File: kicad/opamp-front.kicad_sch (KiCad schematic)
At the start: 84 parts, among them J1 B+, J2 SPK, J3 INPUT, J4 GND, J5 B-, J6 GND, Q1 2N5551, Q10 2N2906, Q11 MJL3281C, Q12 2N2904, Q13 MJL1302C, Q2 BD139, Q3 BD140, Q4 BD139, Q5 BD139, Q6 2N5401, Q7 2N5551, Q8 2N5401, Q9 BD140, U1 LM4562

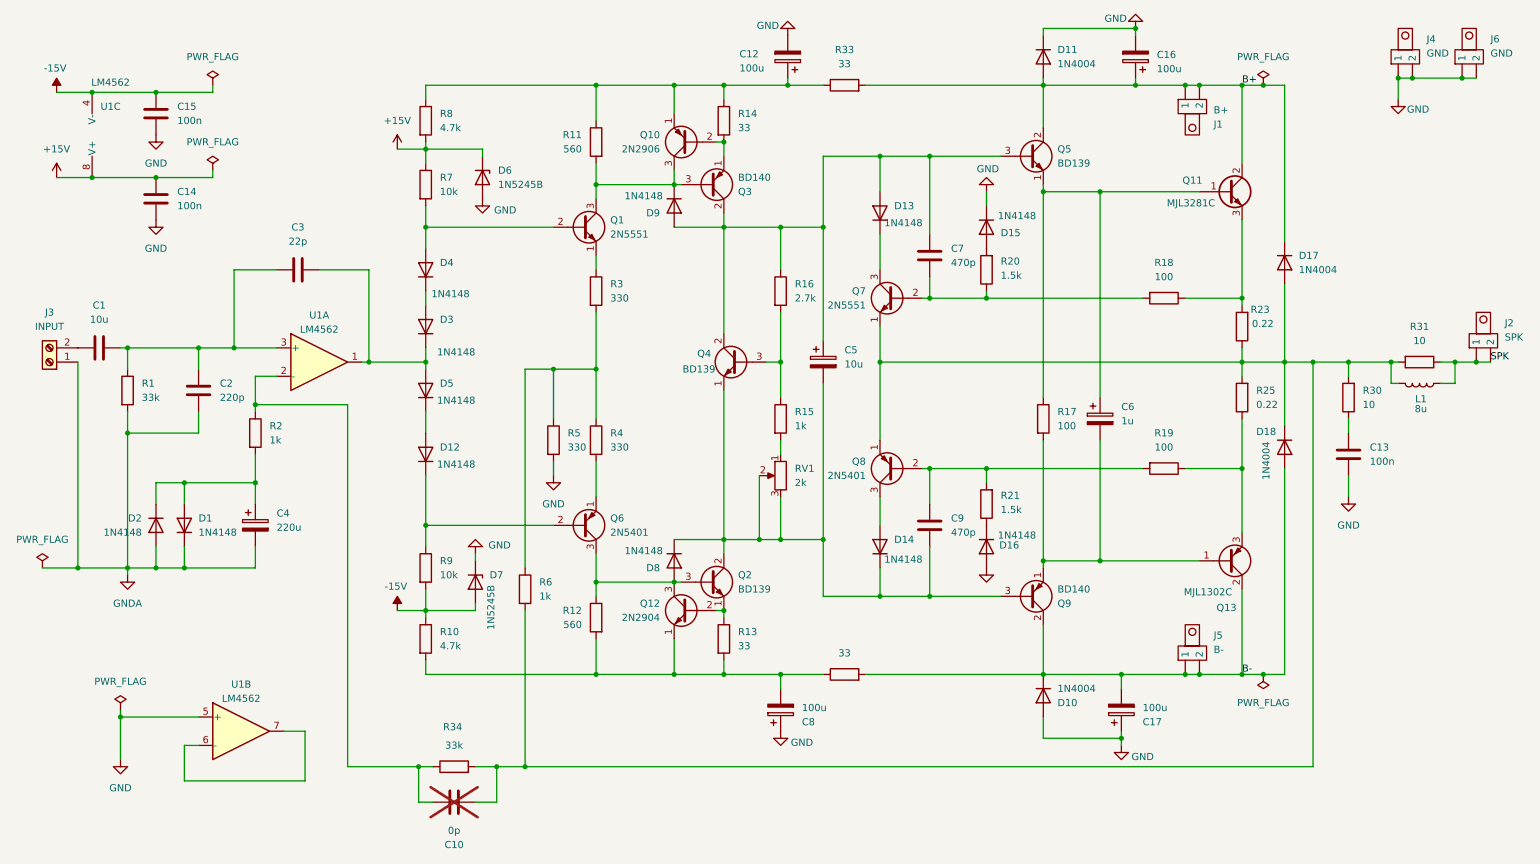
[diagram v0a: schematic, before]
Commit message: Restored after rebase mishap
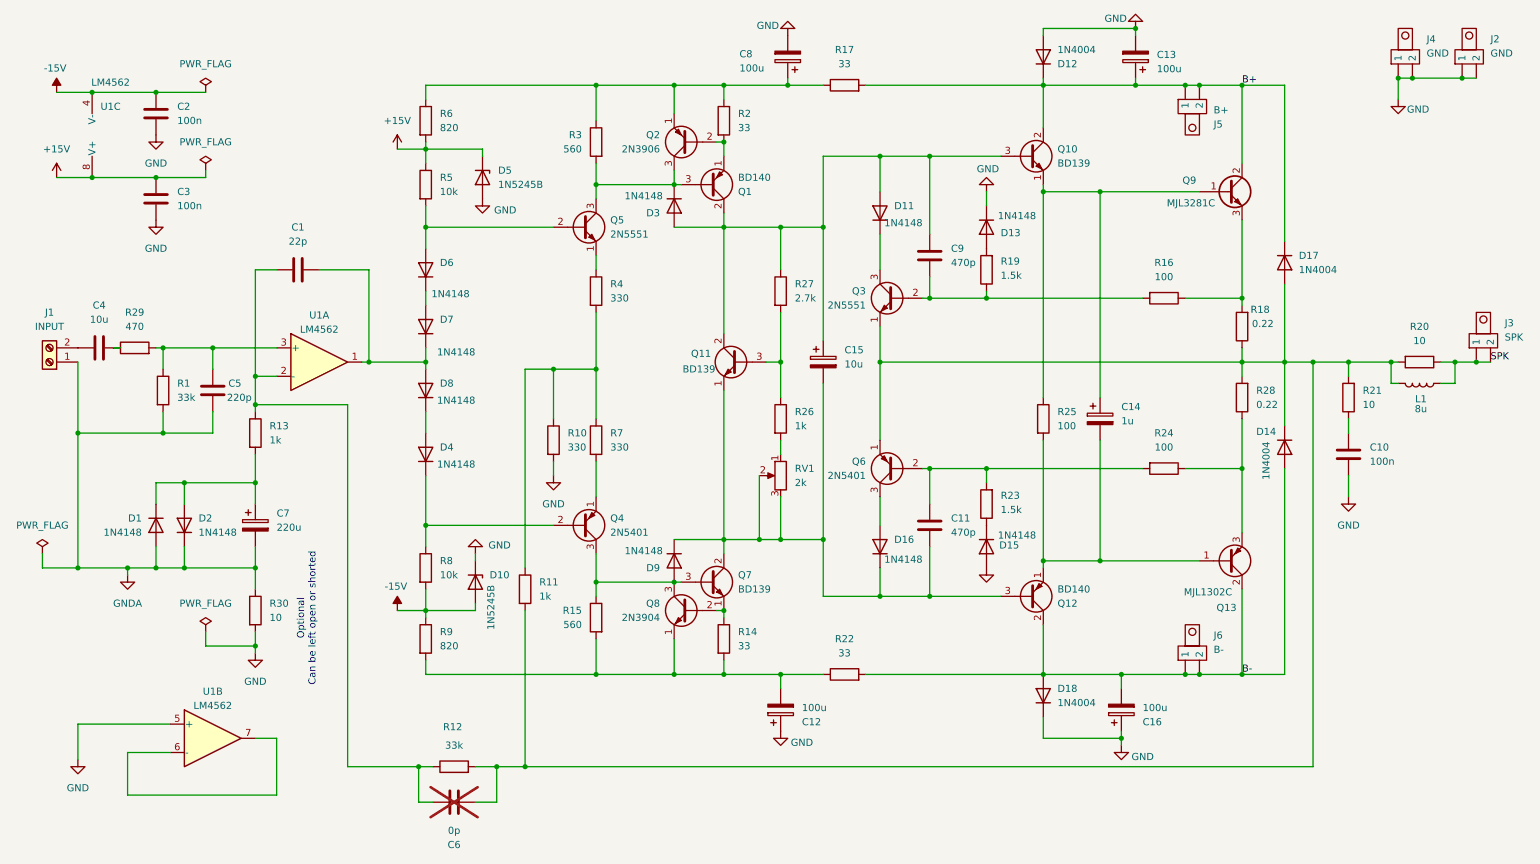
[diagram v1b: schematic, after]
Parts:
- added R29: 470, Resistor_THT:R_Axial_DIN0204_L3.6mm_D1.6mm_P7.62mm_Horizontal, symbol Device:R
- added R30: 10, Resistor_THT:R_Axial_DIN0204_L3.6mm_D1.6mm_P7.62mm_Horizontal, symbol Device:R
- Q2: renamed from Q10; value 2N2906 -> 2N3906
- Q8: renamed from Q12; value 2N2904 -> 2N3904
- R6: renamed from R8; value 4.7k -> 820
- R9: renamed from R10; value 4.7k -> 820
- renumbered C3 to C1, C13 to C10, C9 to C11, C8 to C12, C16 to C13, C6 to C14, C5 to C15, C17 to C16, C15 to C2, C14 to C3, C1 to C4, C2 to C5, C10 to C6, C4 to C7, C12 to C8, C7 to C9, D2 to D1, D7 to D10, D13 to D11, D11 to D12, D15 to D13, D18 to D14, D16 to D15, D14 to D16, D10 to D18, D1 to D2, D9 to D3, D12 to D4, D6 to D5, D4 to D6, D3 to D7, D5 to D8, D8 to D9, J3 to J1, J6 to J2, J2 to J3, J1 to J5, J5 to J6, Q3 to Q1, Q5 to Q10, Q4 to Q11, Q9 to Q12, Q7 to Q3, Q6 to Q4, Q1 to Q5, Q8 to Q6, Q2 to Q7, Q11 to Q9, R5 to R10, R6 to R11, R34 to R12, R2 to R13, R13 to R14, R12 to R15, R18 to R16, R33 to R17, R23 to R18, R20 to R19, R14 to R2, R31 to R20, R30 to R21, R32 to R22, R21 to R23, R19 to R24, R17 to R25, R15 to R26, R16 to R27, R25 to R28, R11 to R3, R3 to R4, R7 to R5, R4 to R7, R9 to R8
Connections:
- net B+: now also D12.1 (K); no longer D12.2 (A)
- net B-: now also D18.2 (A); no longer D18.1 (K)
- net GND: now also D12.2 (A), D18.1 (K), R30.2; no longer D12.1 (K), D18.2 (A)
- net GNDA: now also R30.1
- net at C5.1, R1.1, U1.3 (+): now also R29.2; no longer C1.1, C4.2
- net at C6.1, R12.1, R13.1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: now also C1.1
- new net: C4.2, R29.1
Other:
- note added: "Optional Can be left open or shorted"
- moved on the sheet: C5, R1

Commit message: WIP
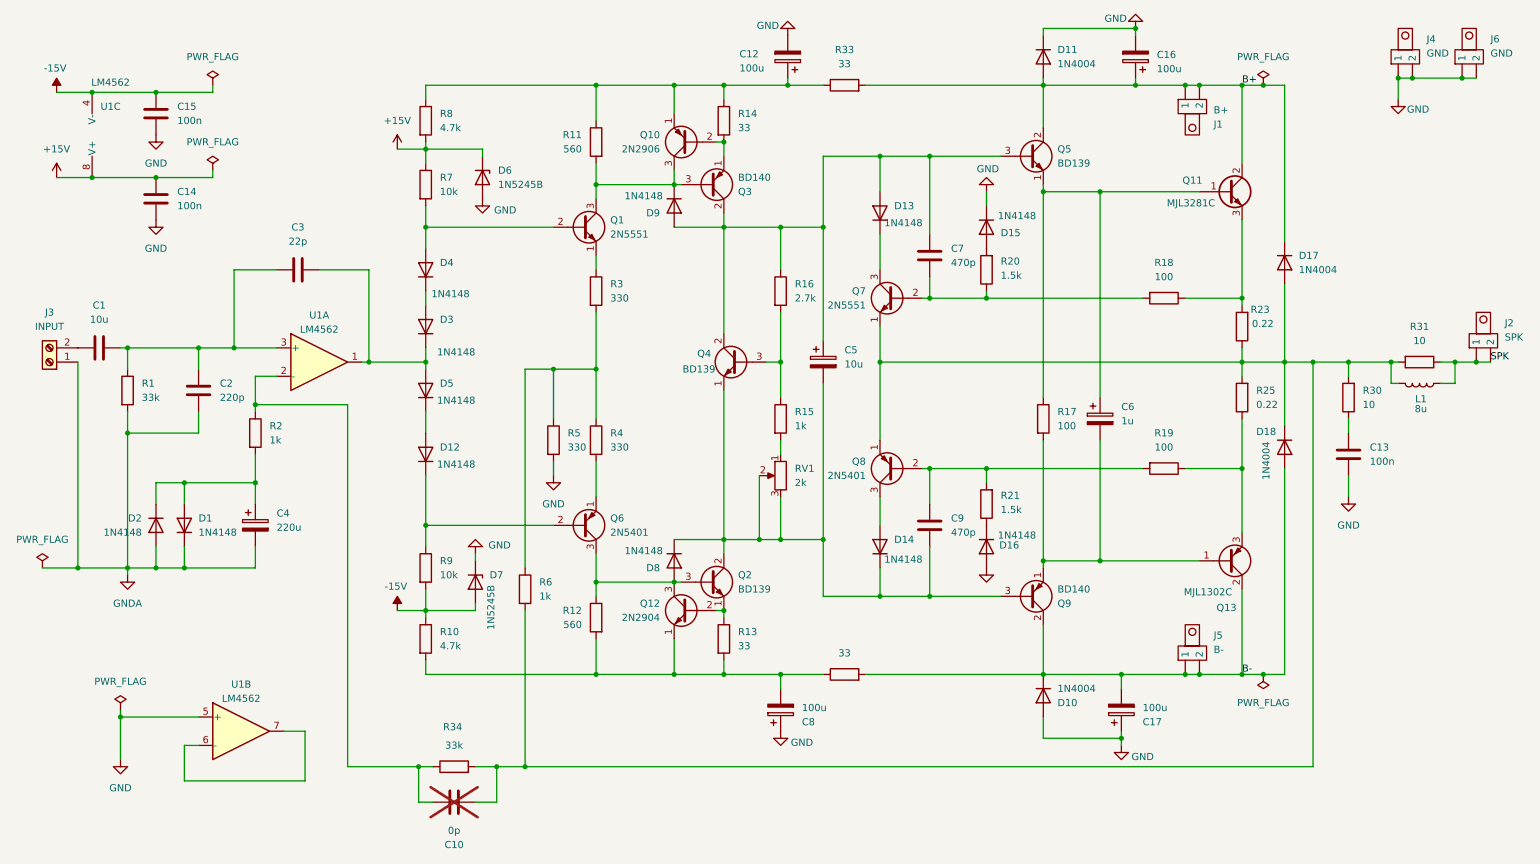
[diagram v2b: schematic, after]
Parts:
- removed R29: 470, Resistor_THT:R_Axial_DIN0204_L3.6mm_D1.6mm_P7.62mm_Horizontal, symbol Device:R
- removed R30: 10, Resistor_THT:R_Axial_DIN0204_L3.6mm_D1.6mm_P7.62mm_Horizontal, symbol Device:R
- Q10: renamed from Q2; value 2N3906 -> 2N2906
- Q12: renamed from Q8; value 2N3904 -> 2N2904
- R10: renamed from R9; value 820 -> 4.7k
- R8: renamed from R6; value 820 -> 4.7k
- renumbered C4 to C1, C6 to C10, C8 to C12, C10 to C13, C3 to C14, C2 to C15, C13 to C16, C16 to C17, C5 to C2, C1 to C3, C7 to C4, C15 to C5, C14 to C6, C9 to C7, C12 to C8, C11 to C9, D2 to D1, D18 to D10, D12 to D11, D4 to D12, D11 to D13, D16 to D14, D13 to D15, D15 to D16, D14 to D18, D1 to D2, D7 to D3, D6 to D4, D8 to D5, D5 to D6, D10 to D7, D9 to D8, D3 to D9, J5 to J1, J3 to J2, J1 to J3, J6 to J5, J2 to J6, Q5 to Q1, Q9 to Q11, Q7 to Q2, Q1 to Q3, Q11 to Q4, Q10 to Q5, Q4 to Q6, Q3 to Q7, Q6 to Q8, Q12 to Q9, R3 to R11, R15 to R12, R14 to R13, R2 to R14, R26 to R15, R27 to R16, R25 to R17, R16 to R18, R24 to R19, R13 to R2, R19 to R20, R23 to R21, R18 to R23, R28 to R25, R4 to R3, R21 to R30, R20 to R31, R22 to R32, R17 to R33, R12 to R34, R7 to R4, R10 to R5, R11 to R6, R5 to R7, R8 to R9
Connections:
- net B+: now also D11.2 (A); no longer D11.1 (K)
- net B-: now also D10.1 (K); no longer D10.2 (A)
- net GND: now also D10.2 (A), D11.1 (K); no longer D10.1 (K), D11.2 (A)
- net at C2.1, R1.1, U1.3 (+): now also C1.2, C3.1
- net at C10.1, R2.1, R34.1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: no longer C3.1
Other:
- note removed: "Optional Can be left open or shorted"
- moved on the sheet: C2, R1
